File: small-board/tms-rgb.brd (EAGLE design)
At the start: 54.4 x 17.6 mm, 39 parts, among them J1 Pads, U1 CD74HC4053PWR, U100 TMS992XA, U2 TS5A4597DCKR, U3 LM1881MX/NOPB, U4 MAX4395EUD, U5 SN74LVC2G17DCKR, U6 LMH1251MT/NOPB, U7 THS7374IPWR

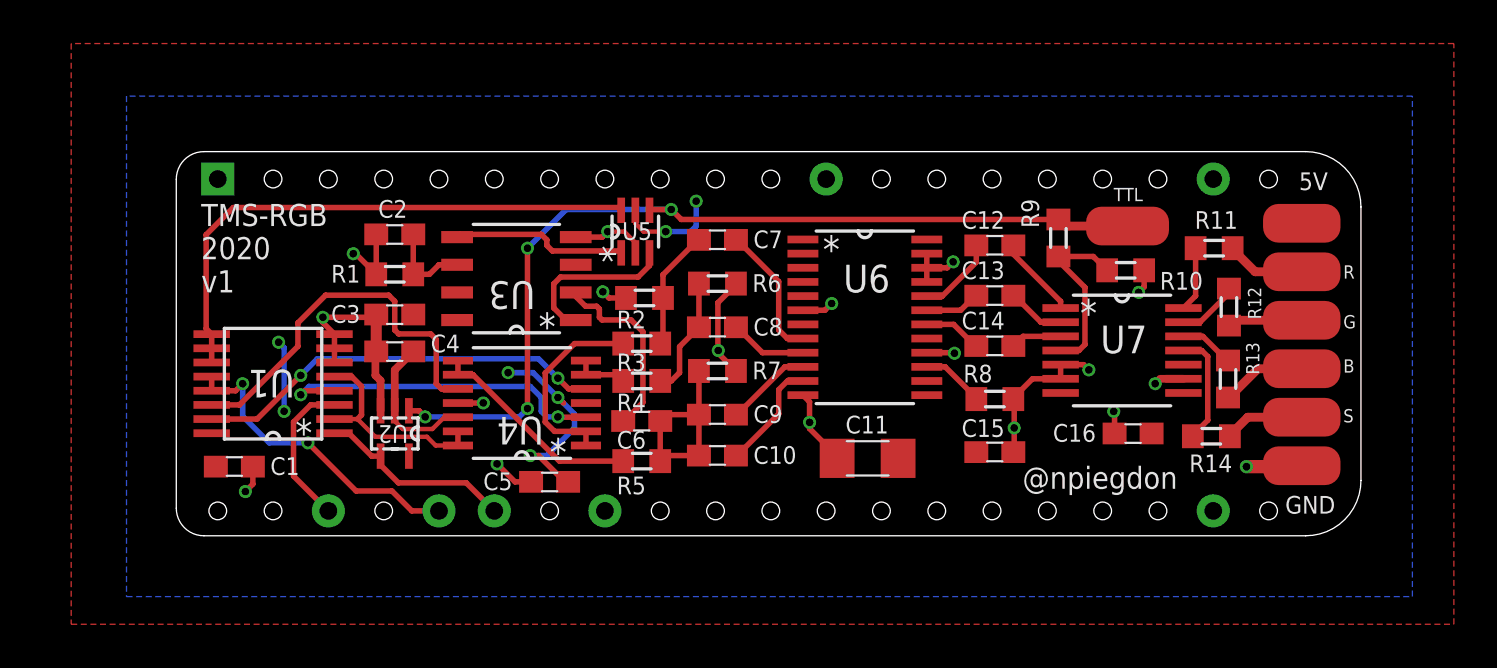
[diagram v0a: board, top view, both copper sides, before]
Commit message: Major layout rework for v2
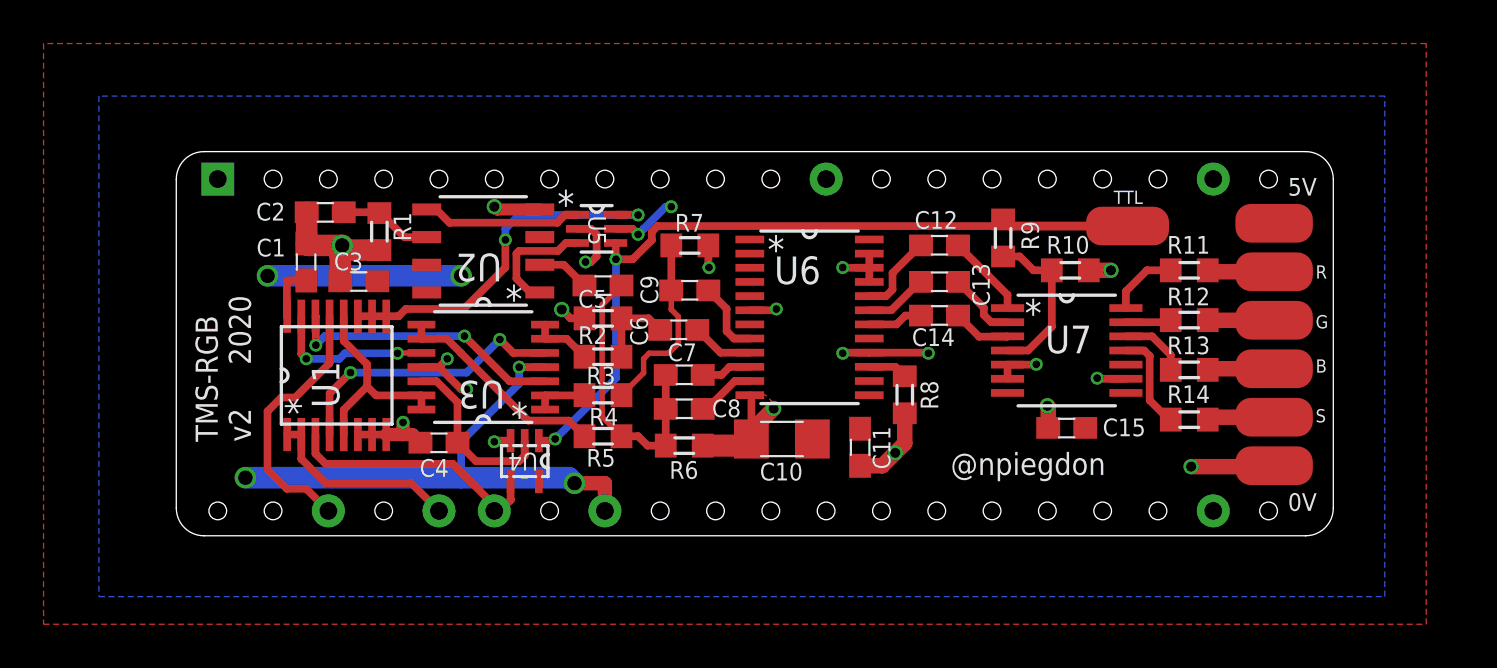
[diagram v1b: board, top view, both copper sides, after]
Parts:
- removed C16: 100nF, tms-rgb:C0603
- C10: value 100nF -> 10uF; device tms-rgb:C0603 -> tms-rgb:C1206
- C11: value 10uF -> 100nF; device tms-rgb:C1206 -> tms-rgb:C0603
- R2: value 150 -> 910
- R3: value 220 -> 680
- R4: value 680 -> 220
- R6: value 910 -> 150
- U2: value TS5A4597DCKR -> LM1881MX/NOPB; device tms-rgb:DCK5 -> tms-rgb:LM1881
- U3: value LM1881MX/NOPB -> MAX4395EUD; device tms-rgb:LM1881 -> tms-rgb:MAX4395
- U4: value MAX4395EUD -> TS5A4597DCKR; device tms-rgb:MAX4395 -> tms-rgb:DCK5
- moved C1 9.96 mm to (5.97, 12.6), turned to 90 degrees
- moved C5 9.34 mm to (19.6, 11.5)
- moved U2 9.32 mm to (14.1, 13.1), turned to 180 degrees
- moved R6 7.60 mm to (23.3, 4.14)
- moved C7 6.39 mm to (23.3, 7.39)
- moved R7 5.90 mm to (23.6, 13.3)
- moved C9 5.84 mm to (23.6, 11.3)
- moved C4 4.66 mm to (12.1, 4.28)
- moved C6 4.52 mm to (23.1, 9.45), turned to 0 degrees
- moved U3 4.34 mm to (14.1, 7.75)
- moved R8 4.14 mm to (33.5, 6.48), turned to 90 degrees
- moved C8 4.05 mm to (23.3, 5.83)
- moved C15 3.48 mm to (40.9, 4.95), turned to 180 degrees
- moved C2 3.35 mm to (6.84, 14.9)
- moved C10 3.06 mm to (27.8, 4.45), turned to 180 degrees
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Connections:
- net B-Y: now also U1.3, U4.4; no longer U1.1, U2.4
- net CSYNC: now also U4.1; no longer U2.1
- net GND: now also C10.2, U2.4, U3.11, U4.3; no longer C16.2, C5.2, U2.3, U3.4, U4.11
- net N$1: now also R4.1, U3.1, U3.2; no longer R3.1, U4.1, U4.2
- net N$10: now also U1.15, U3.10; no longer U1.14, U4.10
- net N$12: now also C9.1, R4.2, R7.2; no longer C7.1, R2.2, R3.2
- net N$13: now also C6.1, R2.2, R3.2; no longer C8.1, R4.2, R6.2
- net N$14: now also C5.1, C7.1, C8.1, R6.2; no longer C10.1, C6.1, C9.1, R7.2
- net N$2: now also R3.1, U3.6, U3.7; no longer R4.1, U4.6, U4.7
- net N$20: now also C5.2, U2.2; no longer C6.2, U3.2
- net N$21: now also C9.2; no longer C7.2
- net N$22: now also C6.2; no longer C8.2
- net N$23: now also C8.2; no longer C10.2
- net N$24: now also C7.2; no longer C9.2
- net N$3: now also U3.8, U3.9; no longer U4.8, U4.9
- net N$4: now also U3.12, U4.2; no longer U2.2, U4.12
- net N$5: now also U2.5; no longer U3.5
- net N$6: now also U2.1; no longer U3.1
- net N$7: now also U2.6; no longer U3.6
- net N$8: now also U1.14, U3.3; no longer U1.4, U4.3
- net N$9: now also U1.4, U3.5; no longer U1.15, U4.5
- net R-Y: now also U1.13; no longer U1.3
- net SAMPLE: now also U1.12, U3.13, U3.14; no longer U1.2, U4.13, U4.14
- net VCC: now also C10.1, U2.8, U3.4, U4.5; no longer C16.1, C5.1, U2.5, U3.8, U4.4
- net Y: now also U1.1, U1.2; no longer U1.12, U1.13
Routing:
- net VCC: track 17.7 -> 39.8 mm
- net N$10: track 17.8 -> 7.45 mm, vias 0 -> 2
- net BURST: track 25.6 -> 16.9 mm, vias 0 -> 2
- net CSYNC: track 42.7 -> 35.5 mm, vias 4 -> 2
- net N$1: track 9.09 -> 2.47 mm
- net N$20: track 8.67 -> 2.45 mm
- net N$9: track 18.9 -> 13.1 mm
- net Y: track 14.5 -> 9.08 mm, vias 2 -> 0
- net R-Y: track 6.95 -> 12.2 mm
- net N$14: track 9.51 -> 13.1 mm
- net B-Y: track 9.06 -> 12.1 mm
- net N$12: track 5.53 -> 8.61 mm
- net N$8: track 15.8 -> 12.9 mm
- net N$21: track 6.25 -> 3.43 mm
- net N$23: track 5.15 -> 2.69 mm
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- added copper zone on layer 1, net GND
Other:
- board size 54.4 x 17.6 mm -> 53.1 x 17.6 mm
- board text added: "0V"
- board text added: "TMS-RGB v2 2020"
- board text removed: "GND"
- board text removed: "TMS-RGB 2020 v1"
